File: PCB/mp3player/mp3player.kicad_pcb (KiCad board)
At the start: 2 copper layers, 60 x 85.5 mm, 70 parts, among them J1 AudioJack3, J2 Battery, J3 USB_C, J4 Micro_SD_Card, J5 TFT SPI, SW1 Play, SW10 Power_sw, SW11 Next, SW12 Prev, SW2 Trk Prev, SW3 Trk Next, SW4 Mode Prev, SW5 Mode Next, SW6 Eq, SW7 Power, SW8 RESET, SW9 BOOT, U1 ESP32-S3-WROOM-1, U2 ES8388, U3 AP2112K-3.3, U4 MCP73831-2-OT, U5 USBLC6-2SC6

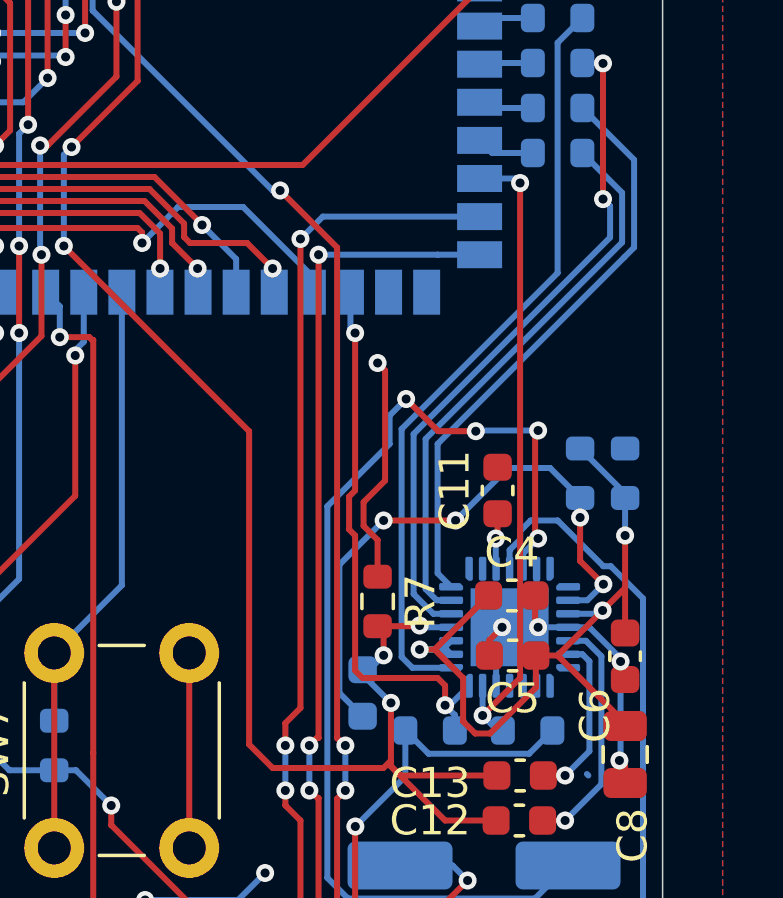
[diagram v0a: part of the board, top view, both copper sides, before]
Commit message: cont
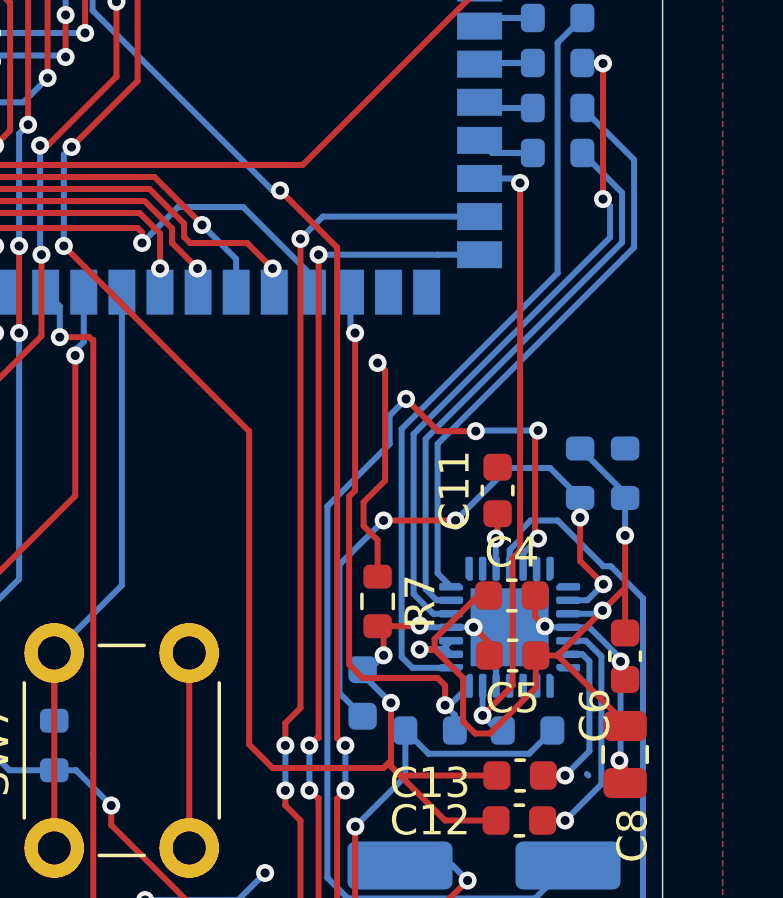
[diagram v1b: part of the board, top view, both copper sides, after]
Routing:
- net AU_GND: track 119.6 -> 121.7 mm
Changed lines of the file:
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@@
 	)
 	(segment
+		(start 237.400001 114.199999)
+		(end 237.400001 114.549999)
+		(width 0.2)
+		(layer "F.Cu")
+		(net "VDD_CODEC")
+	)
+	(segment
+		(start 239.2 112.75)
+		(end 238.85 112.75)
+		(width 0.2)
+		(layer "F.Cu")
+		(net "VDD_CODEC")
+	)
+	(segment
 		(start 241.5 114.75)
 		(end 243 113.25)
@@
 	)
 	(segment
-		(start 243.75 114)
-		(end 243.75 112.5)
+		(start 238.85 112.75)
+		(end 237.400001 114.199999)
 		(width 0.2)
 		(layer "F.Cu")
@@
 	)
 	(segment
-		(start 239.2 112.75)
-		(end 237.400001 114.549999)
+		(start 243.75 114)
+		(end 243.75 112.5)
 		(width 0.2)
 		(layer "F.Cu")
@@
 	)
 	(segment
-		(start 239.225 114.75)
-		(end 239.225 114.234281)
-		(width 0.2)
-		(layer "F.Cu")
-		(net "AU_GND")
-	)
-	(segment
 		(start 243.75 119)
 		(end 243.75 118.44)
@@
 	)
 	(segment
+		(start 239.225 114.337032)
+		(end 238.697063 113.809095)
+		(width 0.2)
+		(layer "F.Cu")
+		(net "AU_GND")
+	)
+	(segment
 		(start 232 118.5)
 		(end 231.217437 117.717437)
@@
 	)
 	(segment
-		(start 239.225 114.234281)
-		(end 239.65 113.809281)
+		(start 240.75 113.451922)
+		(end 241.075983 113.777905)
 		(width 0.2)
 		(layer "F.Cu")
@@
 	)
 	(segment
-		(start 240.75 113.709281)
-		(end 240.85 113.809281)
+		(start 240.75 112.75)
+		(end 240.75 113.451922)
 		(width 0.2)
 		(layer "F.Cu")
@@
 	)
 	(segment
+		(start 239.225 114.75)
+		(end 239.225 114.337032)
+		(width 0.2)
+		(layer "F.Cu")
+		(net "AU_GND")
+	)
+	(segment
 		(start 186.425 85)
 		(end 186.425 86.5)
@@
 	)
 	(segment
-		(start 240.75 112.75)
-		(end 240.75 113.709281)
-		(width 0.2)
-		(layer "F.Cu")
-		(net "AU_GND")
-	)
-	(segment
 		(start 192.5 80.197056)
 		(end 192.5 79.75)
@@
 	)
 	(via
-		(at 239.65 113.809281)
+		(at 192.5 79.75)
 		(size 0.6)
 		(drill 0.3)
@@
 	)
 	(via
-		(at 192.5 79.75)
+		(at 235.944048 116.329629)
 		(size 0.6)
 		(drill 0.3)
@@
 	)
 	(via
-		(at 235.944048 116.329629)
+		(at 243.56 118.25)
 		(size 0.6)
 		(drill 0.3)
@@
 	)
 	(via
-		(at 243.56 118.25)
+		(at 235.7 114.745679)
 		(size 0.6)
 		(drill 0.3)
@@
 	)
 	(via
-		(at 235.7 114.745679)
+		(at 236.9 113.75)
 		(size 0.6)
 		(drill 0.3)
@@
 	)
 	(via
-		(at 236.9 113.75)
+		(at 225.298528 97.8)
 		(size 0.6)
 		(drill 0.3)
@@
 	)
 	(via
-		(at 240.85 113.809281)
+		(at 243.598812 114.95)
 		(size 0.6)
 		(drill 0.3)
@@
 	)
 	(via
-		(at 225.298528 97.8)
+		(at 238.697063 113.809095)
 		(size 0.6)
 		(drill 0.3)
@@
 	)
 	(via
-		(at 243.598812 114.95)
+		(at 241.075983 113.777905)
 		(size 0.6)
 		(drill 0.3)
@@
 	)
 	(segment
+		(start 237.95 113.809281)
+		(end 239.9 113.809281)
+		(width 0.2)
+		(layer "B.Cu")
+		(net "AU_GND")
+	)
+	(segment
 		(start 243.56 118.25)
 		(end 243.598812 118.211188)
@@
 	(segment
 		(start 240.25 99)
-		(end 240.25 115.5)
+		(end 240.25 111.25)
+		(width 0.2)
+		(layer "F.Cu")
+		(net "/12C_SDA")
+	)
+	(segment
+		(start 240 111.5)
+		(end 240 115.75)
 		(width 0.2)
 		(layer "F.Cu")
@@
 	)
 	(segment
-		(start 240.25 115.5)
+		(start 240.25 111.25)
+		(end 240 111.5)
+		(width 0.2)
+		(layer "F.Cu")
+		(net "/12C_SDA")
+	)
+	(segment
+		(start 240 115.75)
 		(end 239 116.75)
 		(width 0.2)
@@
 	)
 	(segment
-		(start 234.75 110.75)
-		(end 234.55 110.55)
-		(width 0.2)
-		(layer "F.Cu")
-		(net "/12C_SCL")
-	)
-	(segment
-		(start 237.75 116.409281)
-		(end 237.75 115.75)
-		(width 0.2)
-		(layer "F.Cu")
-		(net "/12C_SCL")
-	)
-	(segment
 		(start 237.659281 116.5)
 		(end 237.75 116.409281)
@@
 	)
 	(segment
-		(start 237.5 115.5)
-		(end 235 115.5)
+		(start 234.55 115.05)
+		(end 234.55 109.45)
 		(width 0.2)
 		(layer "F.Cu")
@@
 	)
 	(segment
-		(start 234.75 109.25)
-		(end 234.75 104)
+		(start 234.55 109.45)
+		(end 234.75 109.25)
 		(width 0.2)
 		(layer "F.Cu")
@@
 	)
 	(segment
-		(start 235 115.5)
-		(end 234.75 115.25)
+		(start 237.75 116.409281)
+		(end 237.75 115.75)
 		(width 0.2)
 		(layer "F.Cu")
@@
 	)
 	(segment
-		(start 234.55 110.55)
-		(end 234.55 109.45)
+		(start 235 115.5)
+		(end 234.55 115.05)
 		(width 0.2)
 		(layer "F.Cu")
@@
 	)
 	(segment
-		(start 234.75 115.25)
-		(end 234.75 110.75)
+		(start 234.75 109.25)
+		(end 234.75 104)
 		(width 0.2)
 		(layer "F.Cu")
@@
 	)
 	(segment
-		(start 234.55 109.45)
-		(end 234.75 109.25)
+		(start 237.5 115.5)
+		(end 235 115.5)
 		(width 0.2)
 		(layer "F.Cu")

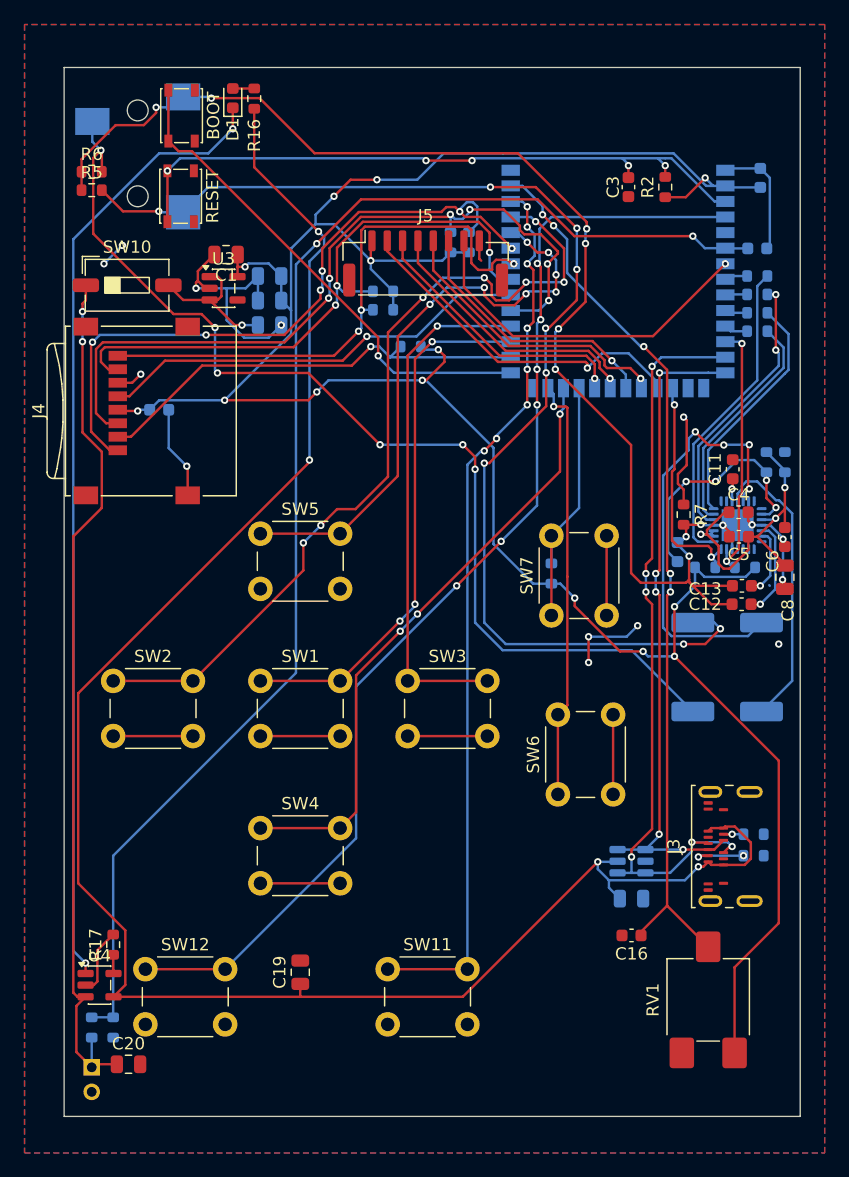
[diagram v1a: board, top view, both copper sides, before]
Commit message: working on drc
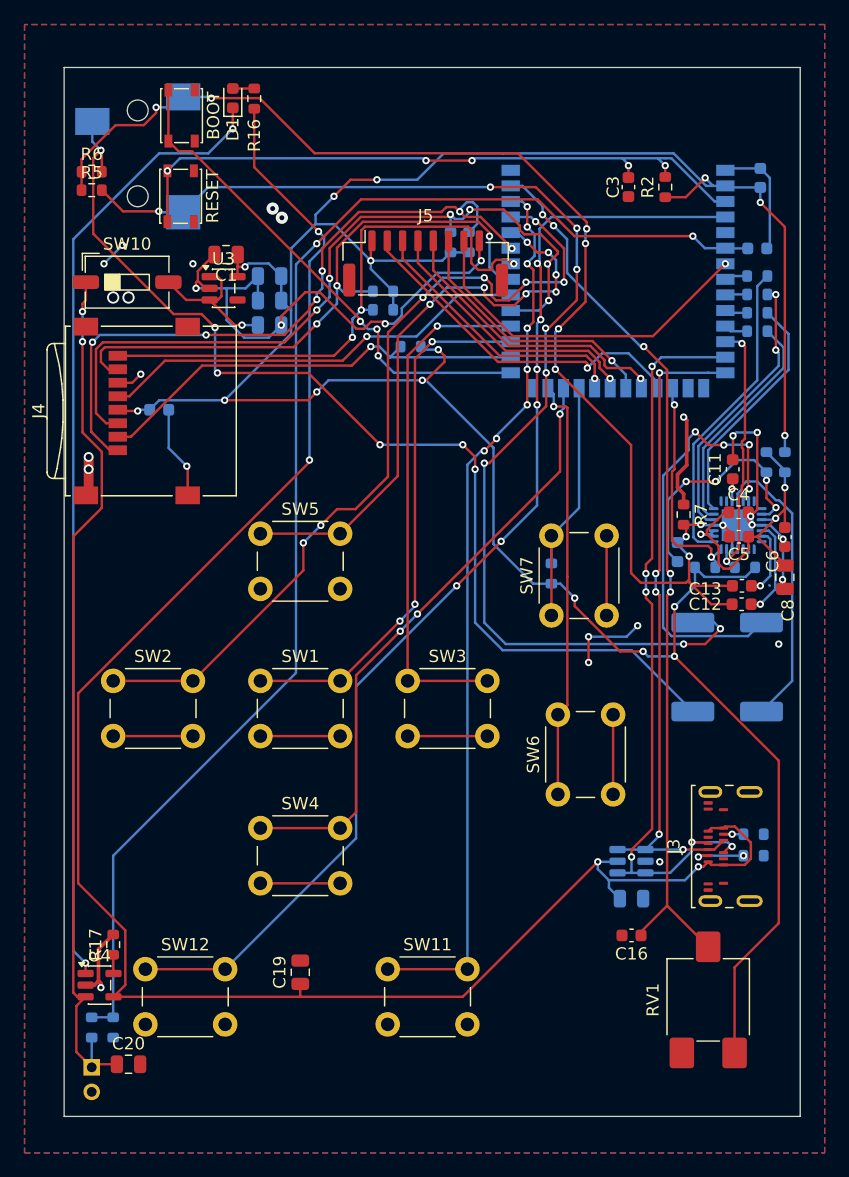
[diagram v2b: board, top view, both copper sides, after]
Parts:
- moved SW10 0.25 mm to (190.1, 94.0)
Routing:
- net GND: track 100.1 -> 126.0 mm, vias 9 -> 20
- net +3V3: track 208.7 -> 231.1 mm, vias 14 -> 16
- net AU_GND: track 121.7 -> 134.1 mm, vias 13 -> 16
- net /IO0: track 40.8 -> 41.2 mm, vias 1 -> 3
